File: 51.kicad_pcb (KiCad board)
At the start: 2 copper layers, 53.5 x 41.5 mm, 11 parts, among them J1 USB_C_Receptacle_USB2.0, J2 Conn_01x11, J3 Conn_01x11, SW1 SW_DPST, U1 STC15W204S-35x-SOP16

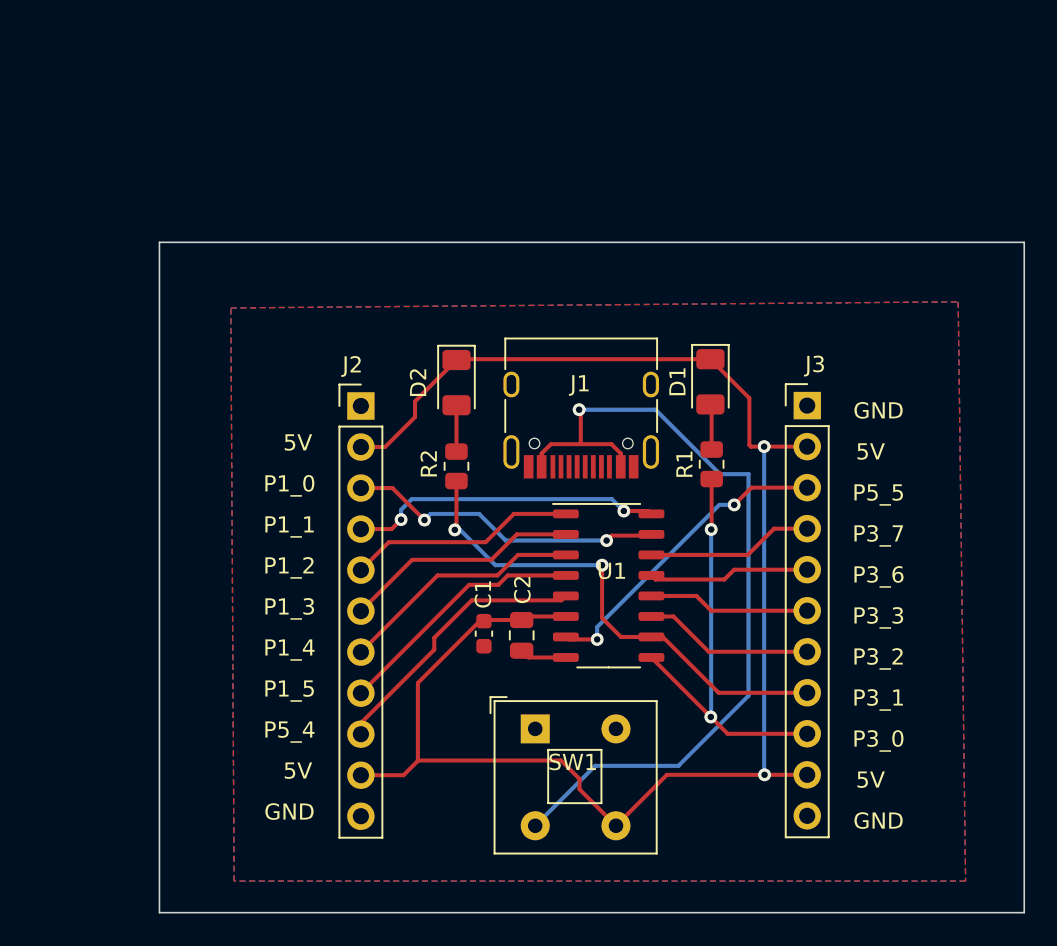
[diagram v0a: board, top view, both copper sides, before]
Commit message: relayout
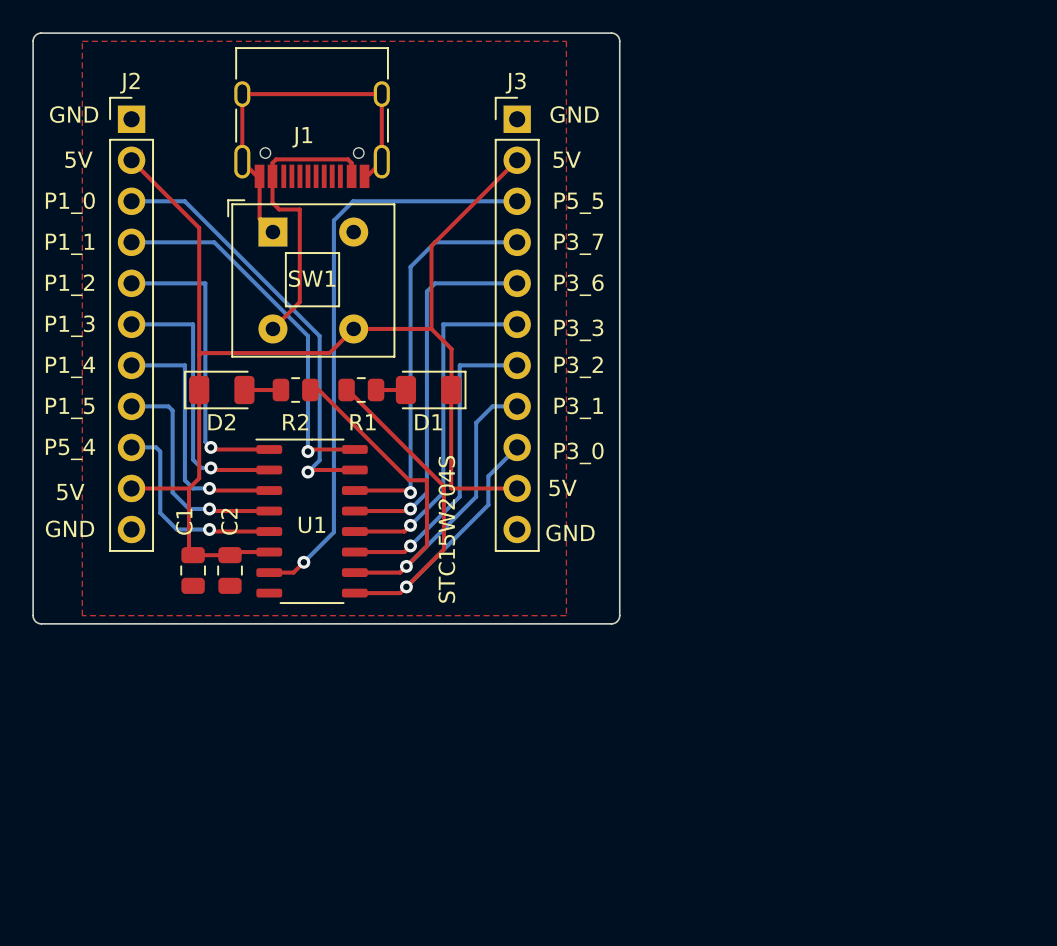
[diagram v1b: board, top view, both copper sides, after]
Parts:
- C1: footprint Capacitor_SMD:C_0603_1608Metric -> Capacitor_SMD:C_0805_2012Metric
- R1, R2: value R -> 10k
- moved SW1 34.8 mm to (93.1, 42.5)
- moved J3 25.2 mm to (108.2, 35.6)
- moved J1 24.5 mm to (95.5, 35.1)
- moved J2 22.7 mm to (84.3, 35.6)
- moved R1 22.2 mm to (98.6, 52.3), turned to 0 degrees
- moved U1 18.8 mm to (95.5, 60.5)
- moved C2 18.5 mm to (90.4, 63.5)
- moved C1 18.4 mm to (88.1, 63.5)
- moved D1 17.5 mm to (102.7, 52.3), turned to 180 degrees
- moved D2 14.5 mm to (89.9, 52.3), turned to 0 degrees
- moved R2 11.0 mm to (94.5, 52.3), turned to 0 degrees
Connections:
- J1 pad A5: GND -> unconnected-(J1-PadA5)
- J1 pad A6: GND -> unconnected-(J1-PadA6)
- J1 pad A7: GND -> unconnected-(J1-PadA7)
- J1 pad A8: GND -> unconnected-(J1-PadA8)
- J1 pad B5: GND -> unconnected-(J1-PadB5)
- J1 pad B6: GND -> unconnected-(J1-PadB6)
- J1 pad B7: GND -> unconnected-(J1-PadB7)
- J1 pad B8: GND -> unconnected-(J1-PadB8)
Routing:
- net +5V: track 51.6 -> 18.3 mm, vias 1 -> 0
- net VCC: track 101.8 -> 77.1 mm, vias 2 -> 0
- net GND: track 0.00 -> 23.7 mm
- net p5_5: track 19.4 -> 36.2 mm, vias 2 -> 1
- net p3_7: track 10.3 -> 24.7 mm, vias 0 -> 1
- net p3_6: track 10.0 -> 23.2 mm, vias 0 -> 1
- net p3_3: track 10.0 -> 21.5 mm, vias 0 -> 1
- net p3_2: track 10.5 -> 19.6 mm, vias 0 -> 1
- net p1_0: track 19.8 -> 26.8 mm, vias 2 -> 1
- net p1_2: track 14.1 -> 18.5 mm, vias 0 -> 1
- net p3_0: track 26.4 -> 30.5 mm, vias 2 -> 1
- net p5_4: track 17.1 -> 12.9 mm, vias 0 -> 1
- net p1_1: track 19.5 -> 23.4 mm, vias 2 -> 1
- net GND1: track 2.91 -> 0.00 mm
- net p1_3: track 14.7 -> 17.2 mm, vias 0 -> 1
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- removed copper zone on B.Cu, net GND1
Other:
- board size 53.5 x 41.5 mm -> 36.3 x 36.6 mm
- board text added: "STC15W204S"
